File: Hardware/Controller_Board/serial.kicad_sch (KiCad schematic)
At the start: 27 parts, among them U10 FT232H, U11 93LC56B, Y2 12MHz

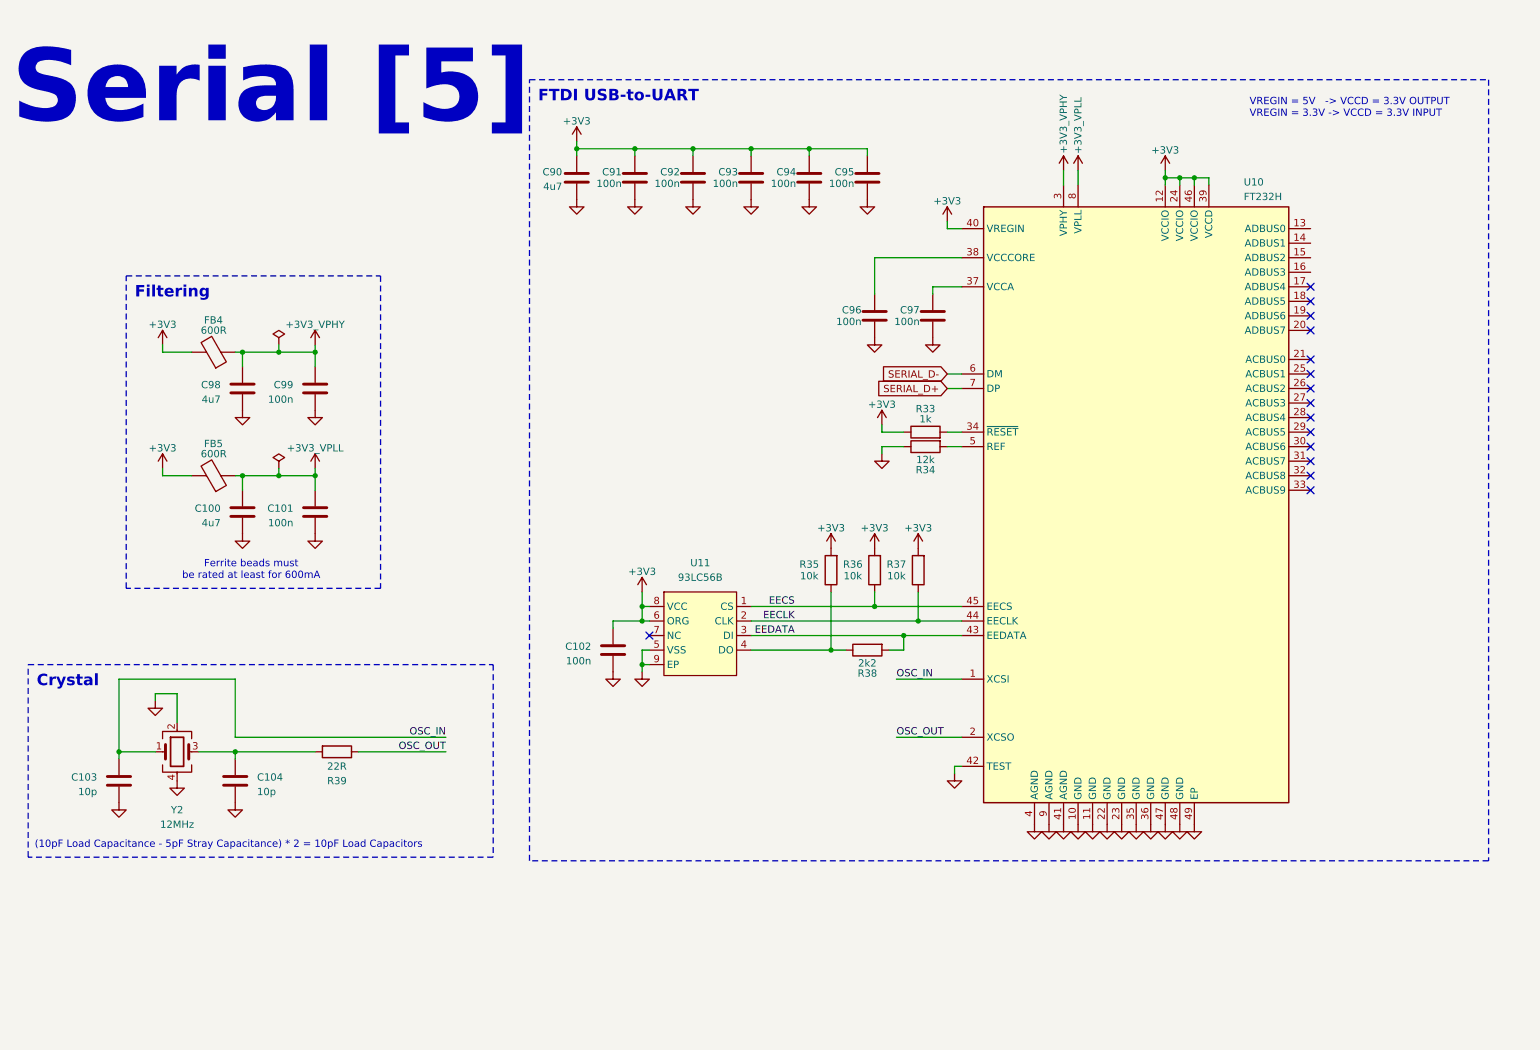
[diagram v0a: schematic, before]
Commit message: Finished schematic design - preparation for review
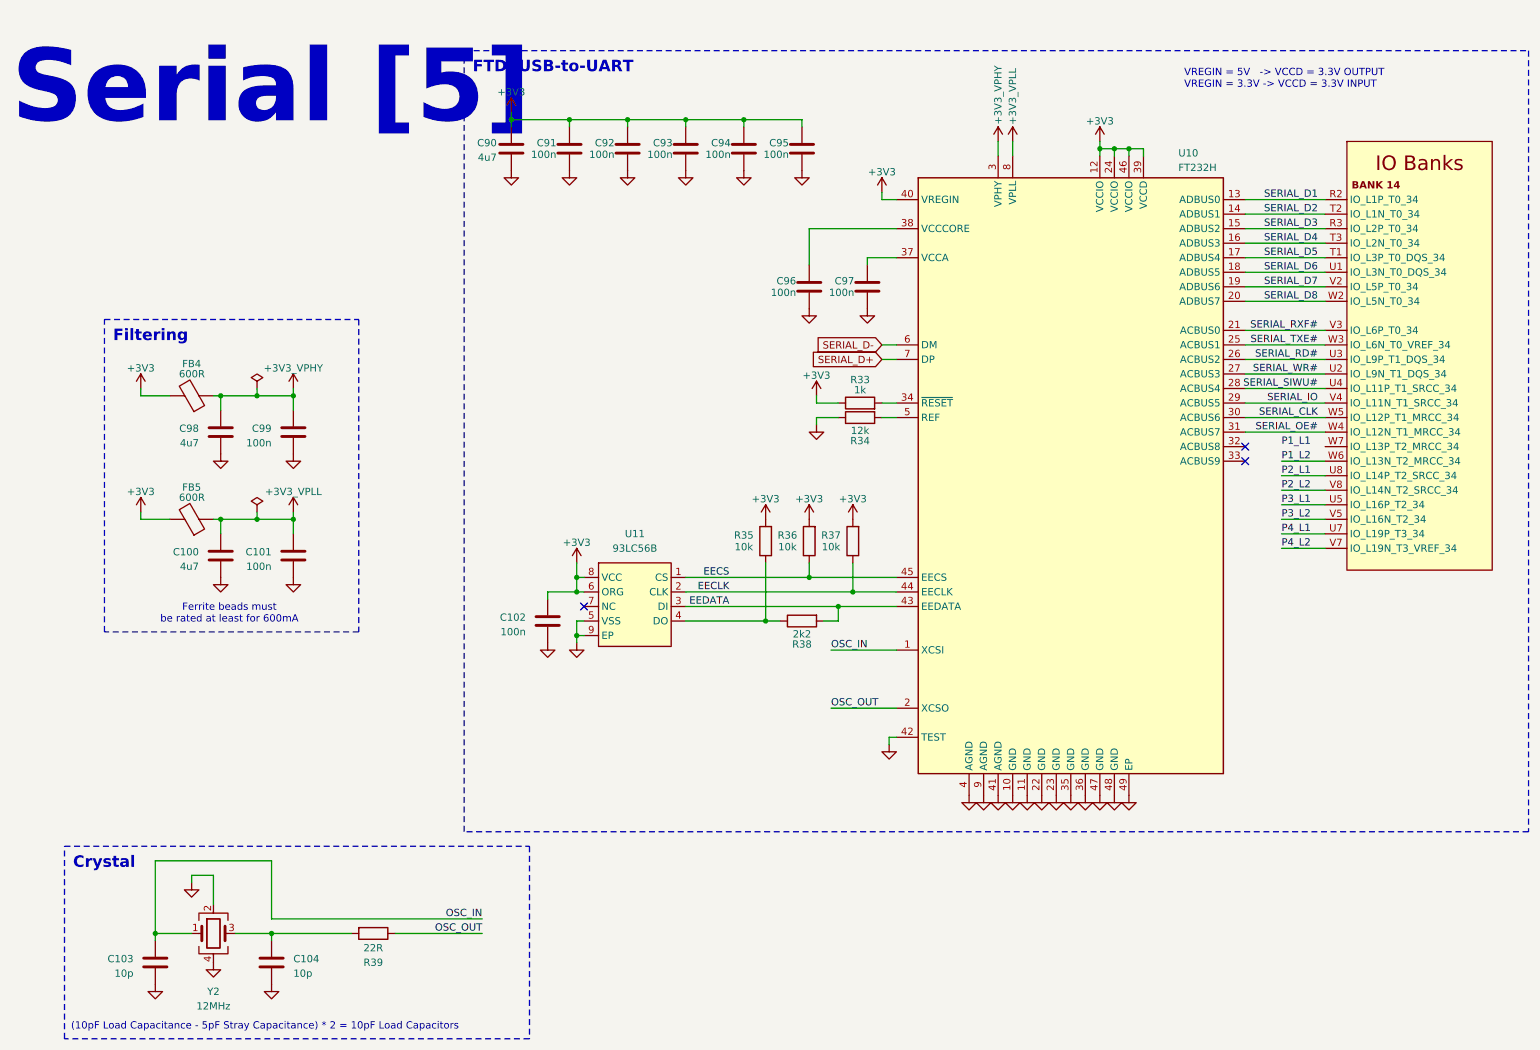
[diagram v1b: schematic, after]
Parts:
- added U6: XC7A35T-CPG236, Package_BGA:Xilinx_CPG236, symbol Custom_VoxLink_Symbols:XC7A35T-CPG236
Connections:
- net SERIAL_D1: now reaches U10.13 (ADBUS0)
- net SERIAL_D1: now also U6.R2 (IO_L1P_T0_34)
- net SERIAL_D2: now reaches U10.14 (ADBUS1)
- net SERIAL_D2: now also U6.T2 (IO_L1N_T0_34)
- net SERIAL_D3: now reaches U10.15 (ADBUS2)
- net SERIAL_D3: now also U6.R3 (IO_L2P_T0_34)
- net SERIAL_D4: now reaches U10.16 (ADBUS3)
- net SERIAL_D4: now also U6.T3 (IO_L2N_T0_34)
- net SERIAL_D5: now reaches U10.17 (ADBUS4)
- net SERIAL_D5: now also U6.T1 (IO_L3P_T0_DQS_34)
- net SERIAL_D6: now reaches U10.18 (ADBUS5)
- net SERIAL_D6: now also U6.U1 (IO_L3N_T0_DQS_34)
- net SERIAL_D7: now reaches U10.19 (ADBUS6)
- net SERIAL_D7: now also U6.V2 (IO_L5P_T0_34)
- net SERIAL_D8: now reaches U10.20 (ADBUS7)
- net SERIAL_D8: now also U6.W2 (IO_L5N_T0_34)
- net SERIAL_RXF#: now reaches U10.21 (ACBUS0)
- net SERIAL_RXF#: now also U6.V3 (IO_L6P_T0_34)
- net SERIAL_TXE#: now reaches U10.25 (ACBUS1)
- net SERIAL_TXE#: now also U6.W3 (IO_L6N_T0_VREF_34)
- net SERIAL_RD#: now reaches U10.26 (ACBUS2)
- net SERIAL_RD#: now also U6.U3 (IO_L9P_T1_DQS_34)
- net SERIAL_WR#: now reaches U10.27 (ACBUS3)
- net SERIAL_WR#: now also U6.U2 (IO_L9N_T1_DQS_34)
- net SERIAL_SIWU#: now reaches U10.28 (ACBUS4)
- net SERIAL_SIWU#: now also U6.U4 (IO_L11P_T1_SRCC_34)
- net SERIAL_IO: now reaches U10.29 (ACBUS5)
- net SERIAL_IO: now also U6.V4 (IO_L11N_T1_SRCC_34)
- net SERIAL_CLK: now reaches U10.30 (ACBUS6)
- net SERIAL_CLK: now also U6.W5 (IO_L12P_T1_MRCC_34)
- net SERIAL_OE#: now reaches U10.31 (ACBUS7)
- net SERIAL_OE#: now also U6.W4 (IO_L12N_T1_MRCC_34)
- new net P1_L2: U6.W6 (IO_L13N_T2_MRCC_34)
- new net P2_L1: U6.U8 (IO_L14P_T2_SRCC_34)
- new net P2_L2: U6.V8 (IO_L14N_T2_SRCC_34)
- new net P3_L1: U6.U5 (IO_L16P_T2_34)
- new net P3_L2: U6.V5 (IO_L16N_T2_34)
- new net P4_L1: U6.U7 (IO_L19P_T3_34)
- new net P4_L2: U6.V7 (IO_L19N_T3_VREF_34)
- no-connect marks 15 -> 3
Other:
- moved on the sheet: C100, C101, C102, C103, C104, C90, C91, C92, C93, C94, C95, C96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
